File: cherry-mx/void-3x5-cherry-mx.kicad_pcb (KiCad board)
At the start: 2 copper layers, 140.5 x 112.5 mm, 82 parts, among them J1 USB_C_Receptacle_PowerOnly_6P, J2 Conn_01x02, J3 Conn_01x02, J4 Conn_01x03

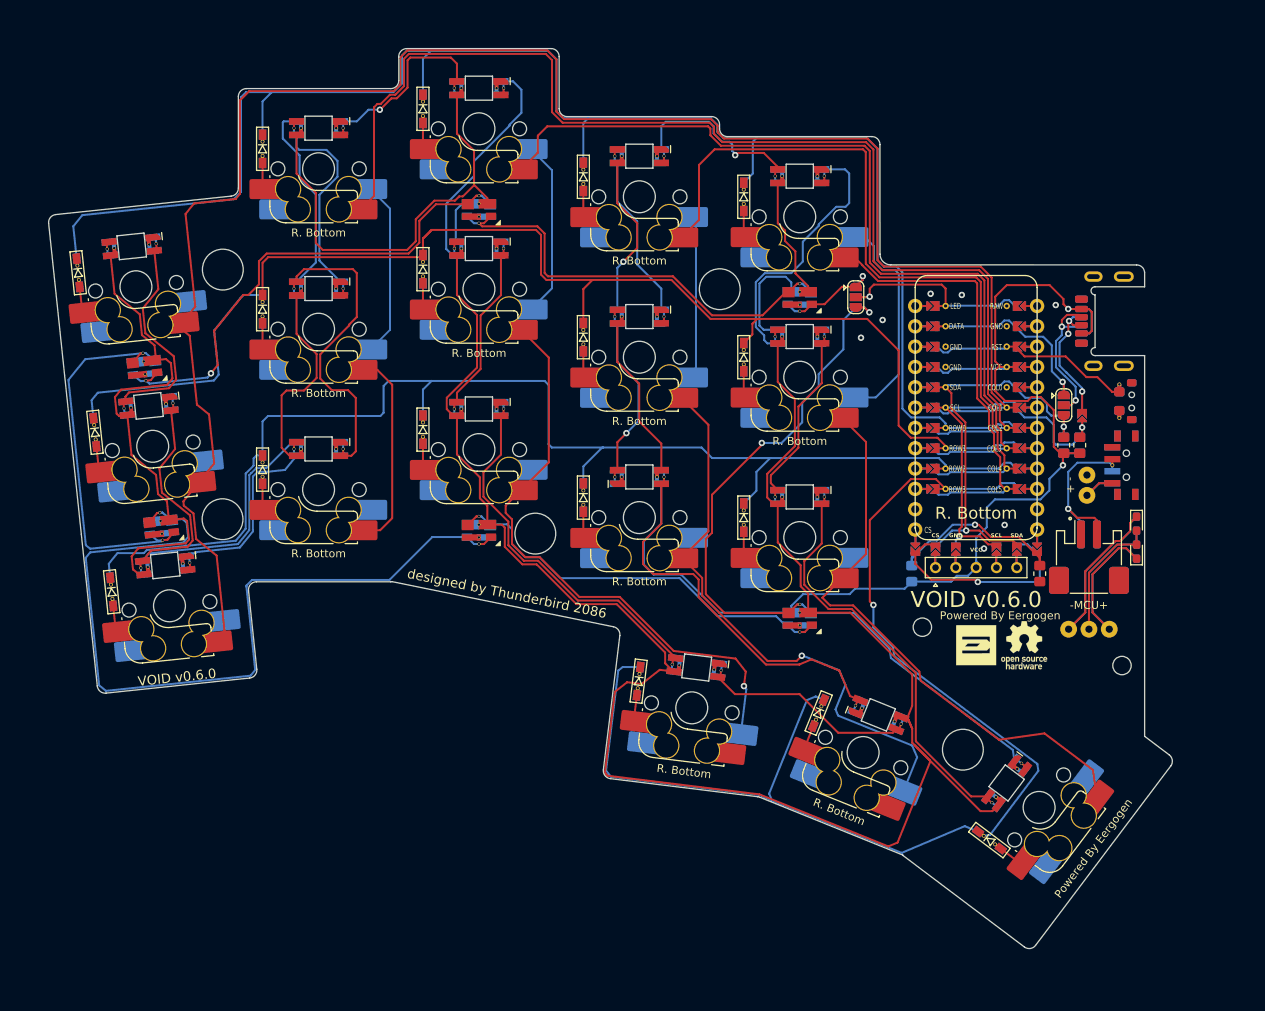
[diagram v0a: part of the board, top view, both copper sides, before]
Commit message: updated PCBs
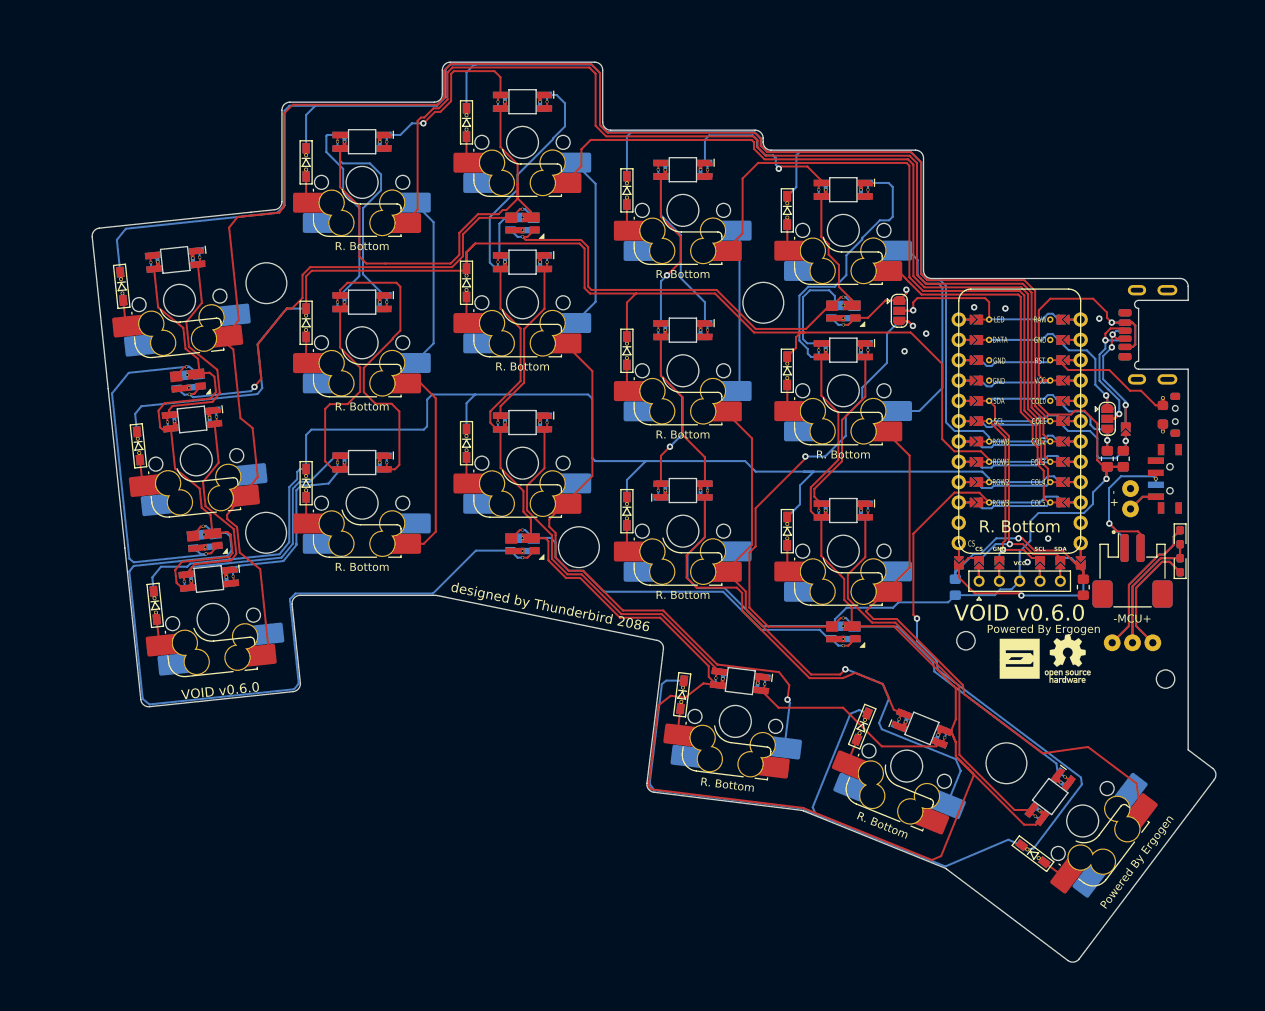
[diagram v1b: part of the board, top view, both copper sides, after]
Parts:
- moved D8 5.70 mm to (133.1, 69.6)
- moved D9 5.70 mm to (133.1, 49.5)
- moved D2 5.70 mm to (92.1, 89.9)
- moved D7 5.70 mm to (133.1, 89.6)
- moved D11 5.70 mm to (153.1, 78.1)
- moved D14 5.70 mm to (173.2, 80.6)
- moved D18 5.70 mm to (203.9, 140.9)
- moved D3 5.70 mm to (90.0, 70.0)
- moved D5 5.70 mm to (113.0, 74.6)
- moved J1 5.70 mm to (219.9, 76.1)
- moved J2 5.70 mm to (216.3, 105.6)
- moved J3 5.70 mm to (216.1, 96.6)
- moved J4 5.70 mm to (216.3, 114.6)
- moved JP1 5.70 mm to (187.2, 73.1)
- moved JP2 5.70 mm to (213.2, 86.6)
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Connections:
- RSW1 pad MP: (no net) -> GND
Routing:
- net Net-(J2-Pin_2): track 20.5 -> 21.1 mm
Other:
- outline, holes or cut-outs redrawn
- board text added: "Powered By Ergogen"
- board text added: "offset: 90, 70 from orign"
- board text removed: "Powered By Eergogen"
- board text removed: "This corner was manually created."
